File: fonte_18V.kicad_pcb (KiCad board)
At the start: 2 copper layers, 100 x 52 mm, 66 parts, among them J101 IN, J102 Conn_01x02, J401 RJ45_Shielded, J402 RJ45_Shielded, Q1 Si2308CDS, Q301 Si2308CDS, U1 LMR16030, U301 LMR16030

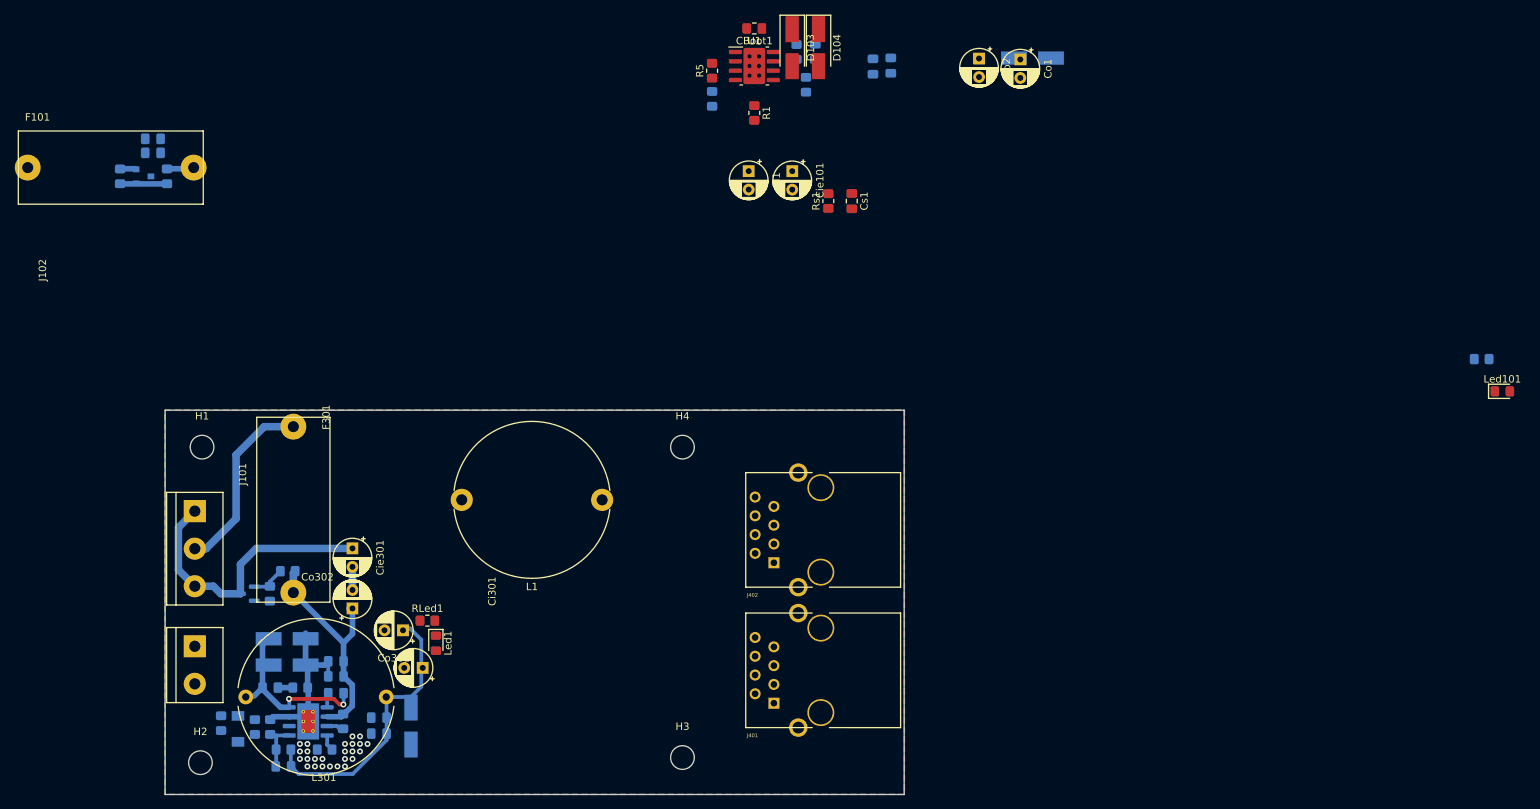
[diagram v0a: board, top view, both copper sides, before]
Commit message: almost finished
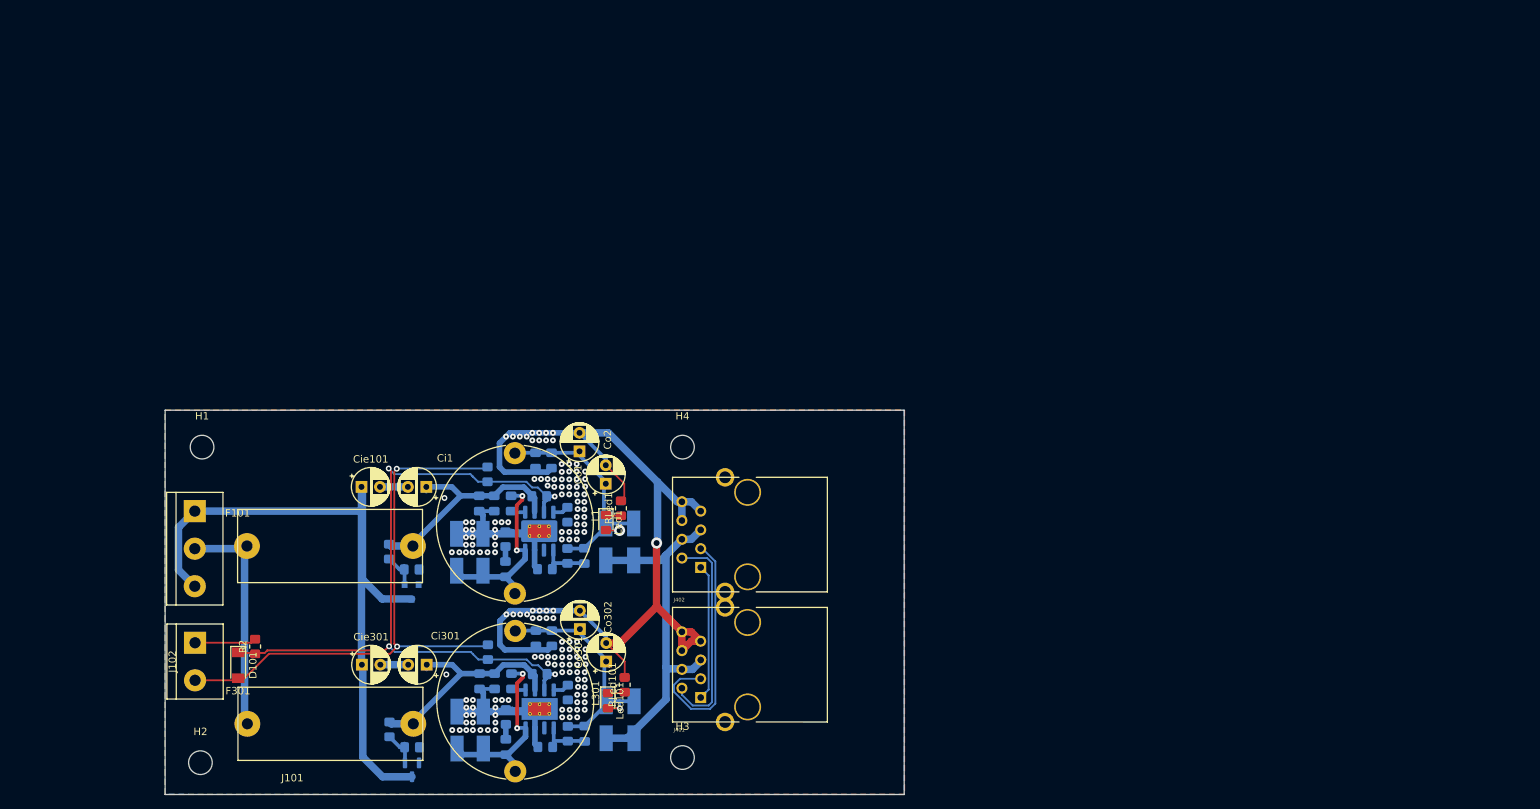
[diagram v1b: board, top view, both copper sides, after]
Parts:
- added D201: MBR340, Diode_SMD:D_SMA_Handsoldering, B.Cu at (85.8, 154.0)
- added D304: MBR340, Diode_SMD:D_SMA_Handsoldering, B.Cu at (85.9, 178.1)
- CBoot1, Cs1, D103, D104, R1, R5, Rs1, U1: moved to B.Cu
- D101, R2, RLed101: moved to F.Cu
- J401, J402: footprint MFP19RJ45:RJ45_YH59_01 -> KicadZeniteSolarLibrary18:RJ45_YH59_01
- moved Led101 128.1 mm to (82.3, 175.5), turned to -90 degrees
- moved RLed101 124.0 mm to (84.6, 173.4), turned to 90 degrees
- moved D102 87.3 mm to (82.0, 154.0), turned to 90 degrees
- moved D104 82.0 mm to (65.4, 155.4), turned to 90 degrees
- moved D103 82.0 mm to (61.8, 155.4), turned to 90 degrees
- moved Co1 80.3 mm to (82.0, 146.2), turned to 90 degrees
- moved Co2 75.8 mm to (78.5, 141.8), turned to 90 degrees
- moved Cff1 75.0 mm to (79.1, 155.9)
- moved Rfbt2 74.9 mm to (76.8, 155.9)
- moved Rfbb1 74.5 mm to (73.8, 157.7), turned to 180 degrees
- moved Cie101 72.3 mm to (49.0, 146.6), turned to 0 degrees
- moved CBoot1 72.2 mm to (69.2, 148.8), turned to -90 degrees
- moved Co3 71.9 mm to (72.5, 143.0)
- moved U1 69.3 mm to (73.0, 152.6), turned to -90 degrees
- moved Co4 68.8 mm to (74.7, 143.0)
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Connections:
- D303 pad 1: /supply2/CAN_18V -> /CAN/CAN_18V
- Led1 pad 2: /CAN/CAN_18V -> /supply1/CAN_18V_DIODE
- Led101 pad 2: /supply2/CAN_18V -> /supply2/CAN_18V_DIODE
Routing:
- net GND: track 23.7 -> 291.8 mm, vias 25 -> 151
- net /EN: track 2.31 -> 97.4 mm, vias 0 -> 4
- net /supply1/GND_IN: track 40.1 -> 99.1 mm
- net /CAN/CAN_18V: track 0.00 -> 50.2 mm
- net /supply1/CAN_18V_DIODE: track 0.00 -> 35.1 mm, vias 0 -> 2
- net Net-(J401-Pad2): track 0.00 -> 28.9 mm
- net Net-(Ci1-Pad1): track 3.45 -> 31.5 mm
- net Net-(CBoot1-Pad1): track 0.00 -> 23.6 mm, vias 0 -> 2
- net Net-(J401-Pad1): track 0.00 -> 20.3 mm
- net Net-(J102-Pad1): track 0.00 -> 8.33 mm
- net /supply1/Feedback: track 0.00 -> 6.57 mm
- net /supply1/IN: track 25.2 -> 31.1 mm
- net Net-(Ci1-Pad2): track 0.00 -> 3.77 mm
- net /supply2/CAN_18V_DIODE: track 37.8 -> 35.1 mm, vias 0 -> 1
- net Net-(Led101-Pad1): track 0.00 -> 2.34 mm
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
